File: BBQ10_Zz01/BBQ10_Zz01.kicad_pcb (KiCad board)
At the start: 2 copper layers, 8 parts, among them J1 USB_C_Receptacle_USB2.0_16P, Q1 AO3401A, U1 E73-2G4M08S1C, U2 USBLC6-2SC6, U3 AP2112K-3.3, U4 MCP73831-5-OT, U5 BBQ10KBD

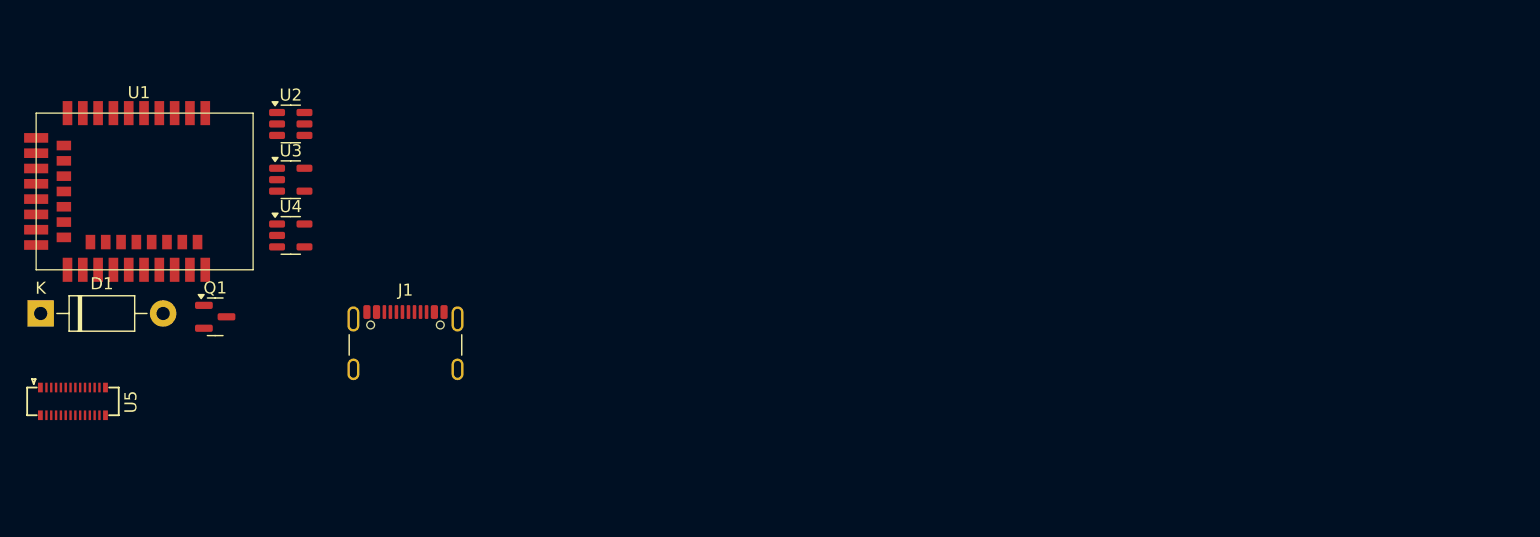
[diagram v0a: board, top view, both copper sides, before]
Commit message: 添加了一些备注，瞎整了一个PCB
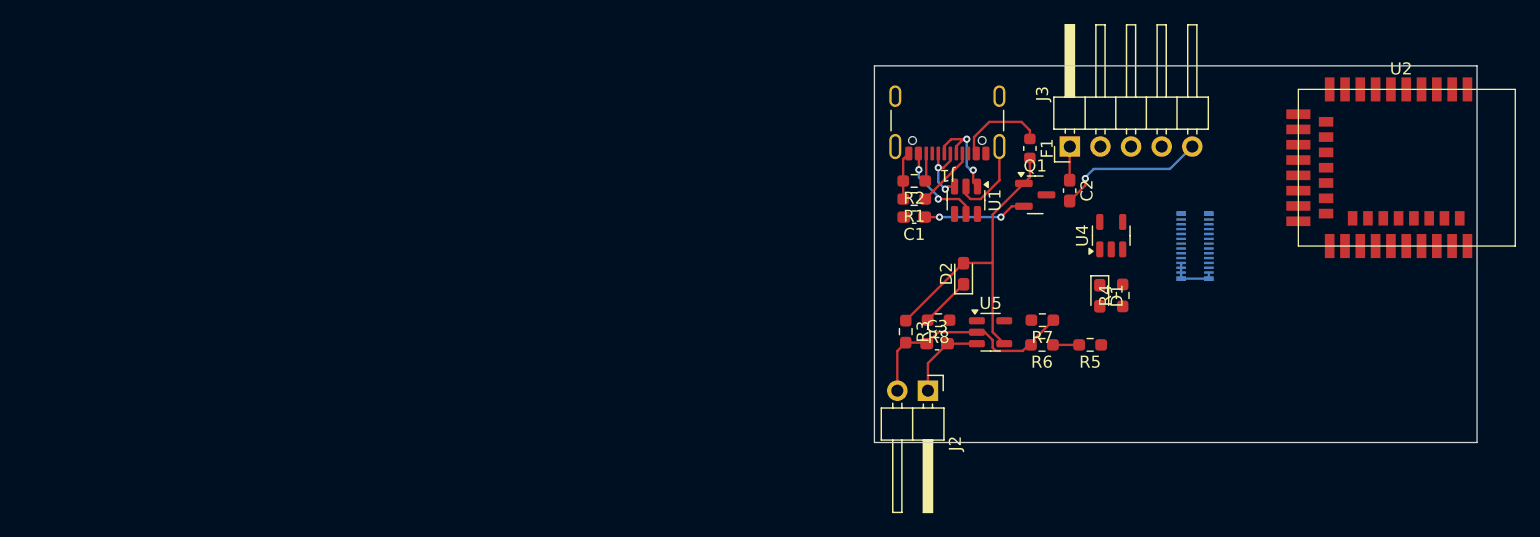
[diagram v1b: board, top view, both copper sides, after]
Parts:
- added C1: C_Small, Capacitor_SMD:C_0603_1608Metric_Pad1.08x0.95mm_HandSolder, F.Cu at (143.3, 62.3)
- added C2: C_Small, Capacitor_SMD:C_0603_1608Metric_Pad1.08x0.95mm_HandSolder, F.Cu at (156.2, 60.1)
- added C3: C_Small, Capacitor_SMD:C_0603_1608Metric_Pad1.08x0.95mm_HandSolder, F.Cu at (145.2, 72.8)
- added D2: LED, LED_SMD:LED_0603_1608Metric_Pad1.05x0.95mm_HandSolder, F.Cu at (147.4, 67.0)
- added F1: Polyfuse_Small, Fuse:Fuse_0603_1608Metric, F.Cu at (152.9, 56.6)
- added J2: Conn_01x02, Connector_PinHeader_2.54mm:PinHeader_1x02_P2.54mm_Horizontal, F.Cu at (144.4, 76.7)
- added J3: Conn_01x05, Connector_PinHeader_2.54mm:PinHeader_1x05_P2.54mm_Horizontal, F.Cu at (156.2, 56.4)
- added R1: R_Small, Resistor_SMD:R_0603_1608Metric_Pad0.98x0.95mm_HandSolder, F.Cu at (143.3, 60.8)
- added R2: R_Small, Resistor_SMD:R_0603_1608Metric_Pad0.98x0.95mm_HandSolder, F.Cu at (143.3, 59.3)
- added R3: R_Small, Resistor_SMD:R_0603_1608Metric_Pad0.98x0.95mm_HandSolder, F.Cu at (142.6, 71.8)
- added R4: R_Small, Resistor_SMD:R_0603_1608Metric_Pad0.98x0.95mm_HandSolder, F.Cu at (160.6, 68.8)
- added R5: R_Small, Resistor_SMD:R_0603_1608Metric_Pad0.98x0.95mm_HandSolder, F.Cu at (157.9, 72.9)
- added R6: R_Small, Resistor_SMD:R_0603_1608Metric_Pad0.98x0.95mm_HandSolder, F.Cu at (153.9, 72.9)
- added R7: R_Small, Resistor_SMD:R_0603_1608Metric_Pad0.98x0.95mm_HandSolder, F.Cu at (153.9, 70.8)
- added R8: R_Small, Resistor_SMD:R_0603_1608Metric_Pad0.98x0.95mm_HandSolder, F.Cu at (145.3, 70.8)
- D1: footprint Diode_THT:D_DO-41_SOD81_P10.16mm_Horizontal -> Diode_SMD:D_0603_1608Metric_Pad1.05x0.95mm_HandSolder
- U1: value E73-2G4M08S1C -> USBLC6-2SC6; footprint nk600:E73(2G4M08S1C) -> Package_TO_SOT_SMD:SOT-23-6
- U2: value USBLC6-2SC6 -> E73-2G4M08S1C; footprint Package_TO_SOT_SMD:SOT-23-6 -> nk600:E73(2G4M08S1C)
- U3: value AP2112K-3.3 -> BBQ10KBD; footprint Package_TO_SOT_SMD:SOT-23-5 -> nk600:BM14B(0.8)-24DS-0.4V(53); moved to B.Cu
- U4: value MCP73831-5-OT -> AP2112K-3.3
- U5: value BBQ10KBD -> MCP73831-5-OT; footprint nk600:BM14B(0.8)-24DS-0.4V(53) -> Package_TO_SOT_SMD:SOT-23-5
- moved D1 87.9 mm to (158.7, 68.8), turned to -90 degrees
- moved U2 84.2 mm to (175.2, 64.7)
- moved U1 77.4 mm to (147.6, 60.9), turned to -90 degrees
- moved U5 76.4 mm to (149.6, 71.8)
- moved U3 75.2 mm to (166.6, 64.7), turned to -90 degrees
- moved Q1 68.8 mm to (153.3, 60.5)
- moved U4 68.1 mm to (159.7, 63.8), turned to 90 degrees
- moved J1 49.4 mm to (146.1, 53.3), turned to 180 degrees
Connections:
- J1 pad A4: Net-(U2-VBUS) -> Net-(U1-VBUS)
- J1 pad A9: Net-(U2-VBUS) -> Net-(U1-VBUS)
- J1 pad B4: Net-(U2-VBUS) -> Net-(U1-VBUS)
- J1 pad B9: Net-(U2-VBUS) -> Net-(U1-VBUS)
- U1 pad 1: unconnected-(U1-P1.11-Pad1) -> Net-(J1-D--PadA7)
- U1 pad 2: unconnected-(U1-P1.10-Pad2) -> Net-(J1-SHIELD)
- U1 pad 3: unconnected-(U1-P0.03-Pad3) -> Net-(J1-D+-PadA6)
- U1 pad 4: unconnected-(U1-AI4-Pad4) -> /D+
- U1 pad 5: unconnected-(U1-GND-Pad5) -> Net-(U1-VBUS)
- U1 pad 6: unconnected-(U1-P1.13-Pad6) -> /D-
- U2 pad 1: Net-(J1-D--PadA7) -> Net-(U2-P1.11)
- U2 pad 2: Net-(J1-SHIELD) -> Net-(U2-P1.10)
- U2 pad 3: Net-(J1-D+-PadA6) -> Net-(U2-P0.03)
- U2 pad 4: /D+ -> Net-(U2-AI4/P0.28)
- U2 pad 5: Net-(U2-VBUS) -> GND
- U2 pad 6: /D- -> Net-(U2-P1.13)
- U3 pad 1: Net-(D1-K) -> GND
- U3 pad 2: GND -> unconnected-(U3-MIC_VDD-Pad2)
- U3 pad 3: Net-(U3-EN) -> unconnected-(U3-MIC-Pad3)
- U3 pad 5: VCC -> GND
- U4 pad 1: Net-(U4-STAT) -> Net-(D1-K)
- U4 pad 3: /VBAT -> Net-(U4-EN)
- U4 pad 4: /VBUS -> unconnected-(U4-NC-Pad4)
- U4 pad 5: Net-(U4-PROG) -> VCC
- U5 pad 1: Net-(U5-GND-Pad1) -> Net-(U5-STAT)
- U5 pad 2: unconnected-(U5-MIC_VDD-Pad2) -> GND
- U5 pad 3: unconnected-(U5-MIC-Pad3) -> /VBAT
- U5 pad 4: unconnected-(U5-AGND-Pad4) -> /VBUS
- U5 pad 5: Net-(U5-GND-Pad1) -> Net-(U5-PROG)
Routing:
- net GND: track 0.00 -> 39.5 mm, vias 0 -> 1
- net /VBUS: track 0.00 -> 26.3 mm
- net Net-(U1-VBUS): track 0.00 -> 15.3 mm, vias 0 -> 2
- net Net-(J1-D--PadA7): track 0.00 -> 8.84 mm, vias 0 -> 2
- net Net-(D1-K): track 0.00 -> 8.61 mm, vias 0 -> 2
- net Net-(J1-SHIELD): track 0.00 -> 7.03 mm
- net /VBAT: track 0.00 -> 7.01 mm
- net Net-(J1-D+-PadA6): track 0.00 -> 5.91 mm, vias 0 -> 2
- net Net-(J1-CC1): track 0.00 -> 5.06 mm
- net Net-(D2-K): track 0.00 -> 4.22 mm
- net VCC: track 0.00 -> 2.80 mm
- net Net-(J1-CC2): track 0.00 -> 2.32 mm
- net /BAT_Level_Check: track 0.00 -> 2.18 mm
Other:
- board outline added: 50 x 31.2 mm
